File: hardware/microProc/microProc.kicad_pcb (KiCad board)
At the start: 2 copper layers, 23 parts, among them J1 POWER, J2 INPUT, J3 OUTPUT, J4 Conn_02x07_Odd_Even, U1 STM32L021K4Tx, U2 BU33SD5WG-TR, U3 MCP4801

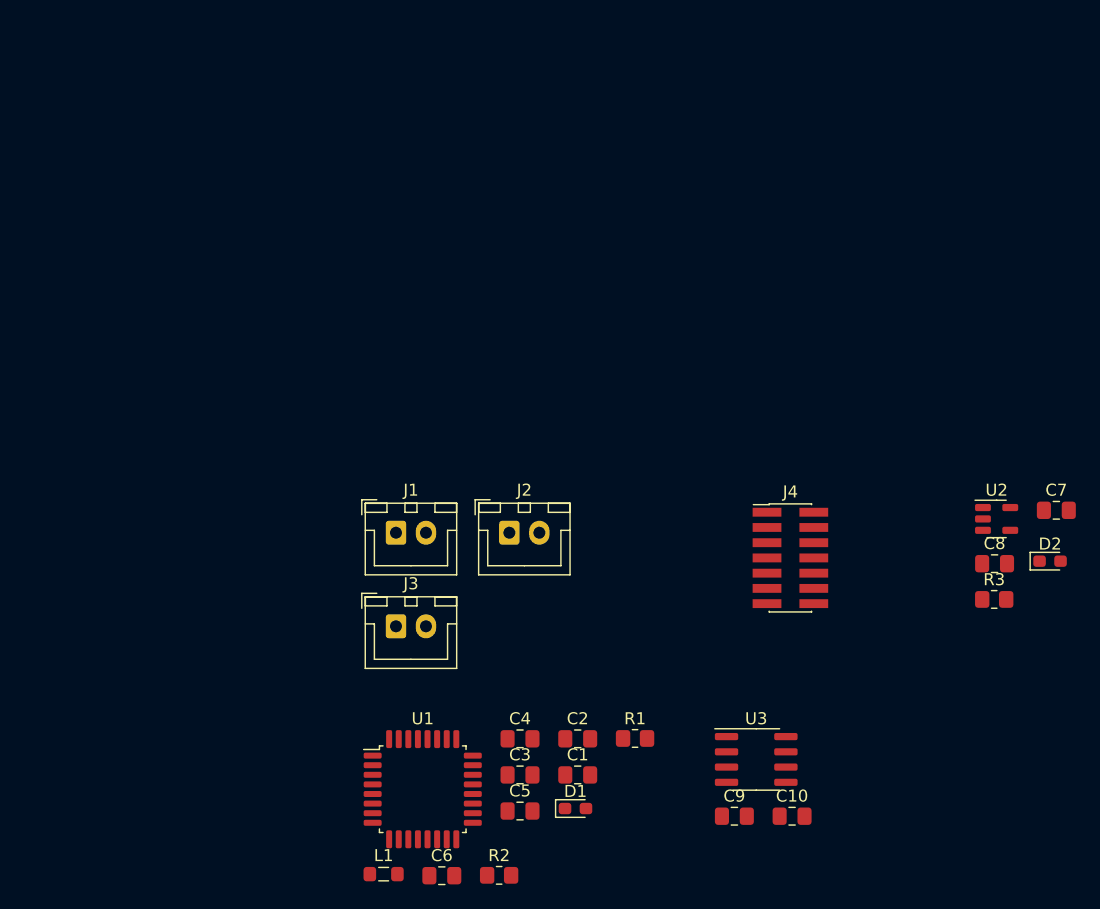
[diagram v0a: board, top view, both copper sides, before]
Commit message: Component placement
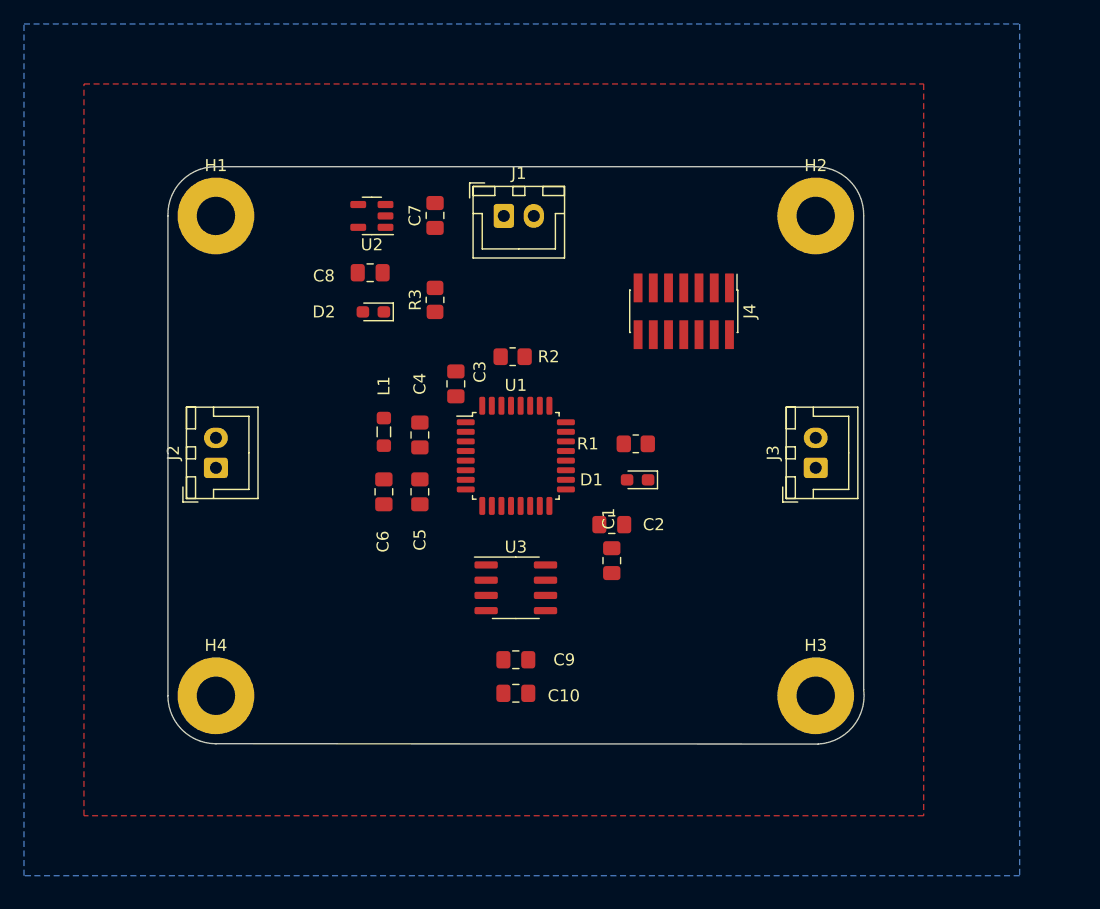
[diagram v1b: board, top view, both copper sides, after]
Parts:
- added H1: MountingHole_Pad, MountingHole:MountingHole_3.2mm_M3_Pad, F.Cu at (107.0, 55.0)
- added H2: MountingHole_Pad, MountingHole:MountingHole_3.2mm_M3_Pad, F.Cu at (157.0, 55.0)
- added H3: MountingHole_Pad, MountingHole:MountingHole_3.2mm_M3_Pad, F.Cu at (157.0, 95.0)
- added H4: MountingHole_Pad, MountingHole:MountingHole_3.2mm_M3_Pad, F.Cu at (107.0, 95.0)
- moved D2 60.1 mm to (120.1, 63.0), turned to 180 degrees
- moved U2 57.9 mm to (120.0, 55.0), turned to 180 degrees
- moved C8 57.4 mm to (119.9, 59.7)
- moved C7 57.3 mm to (125.3, 55.0), turned to 90 degrees
- moved R3 52.9 mm to (125.3, 62.0), turned to 90 degrees
- moved R2 43.2 mm to (131.7, 66.7)
- moved J3 37.4 mm to (157.0, 76.0), turned to 90 degrees
- moved L1 36.9 mm to (121.0, 73.0), turned to 90 degrees
- moved C3 33.0 mm to (127.0, 69.0), turned to 90 degrees
- moved C6 32.4 mm to (121.0, 78.0), turned to -90 degrees
- moved U1 28.9 mm to (132.0, 75.0)
- moved J1 27.9 mm to (131.0, 55.0)
- moved C5 27.9 mm to (124.0, 78.0), turned to -90 degrees
- moved D1 27.9 mm to (142.2, 77.0), turned to 180 degrees
- moved C4 26.7 mm to (124.0, 73.3), turned to 90 degrees
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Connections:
- D1 pad 1: LED_STATUS -> Net-(R1-Pad1)
- D1 pad 2: Net-(D1-Pad2) -> LED_STATUS
- R1 pad 1: Net-(D1-Pad2) -> Net-(R1-Pad1)
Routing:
- added copper zone on B.Cu, net GND
- added copper zone on F.Cu, net GND
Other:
- board outline added: 58 x 48.1 mm
